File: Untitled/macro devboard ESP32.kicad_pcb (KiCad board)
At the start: 4 copper layers, 65.6 x 57.1 mm, 57 parts, among them J1 12402012E212A, J3 Conn_02x04_Odd_Even, J4 Conn_01x02_Pin, Q1 BSS84LT1G, SW1 MX_SW_HS, SW2 1825232-1, SW3 RST, SW6 MX_SW_HS, SW7 MX_SW_HS, SW8 MX_SW_HS, SW9 MX_SW_HS, U1 ESP32-C3-WROOM-02, U2 MCP73831T-2ACI_OT, U3 USBLC6-2SC6, U4 XC6210B332MR

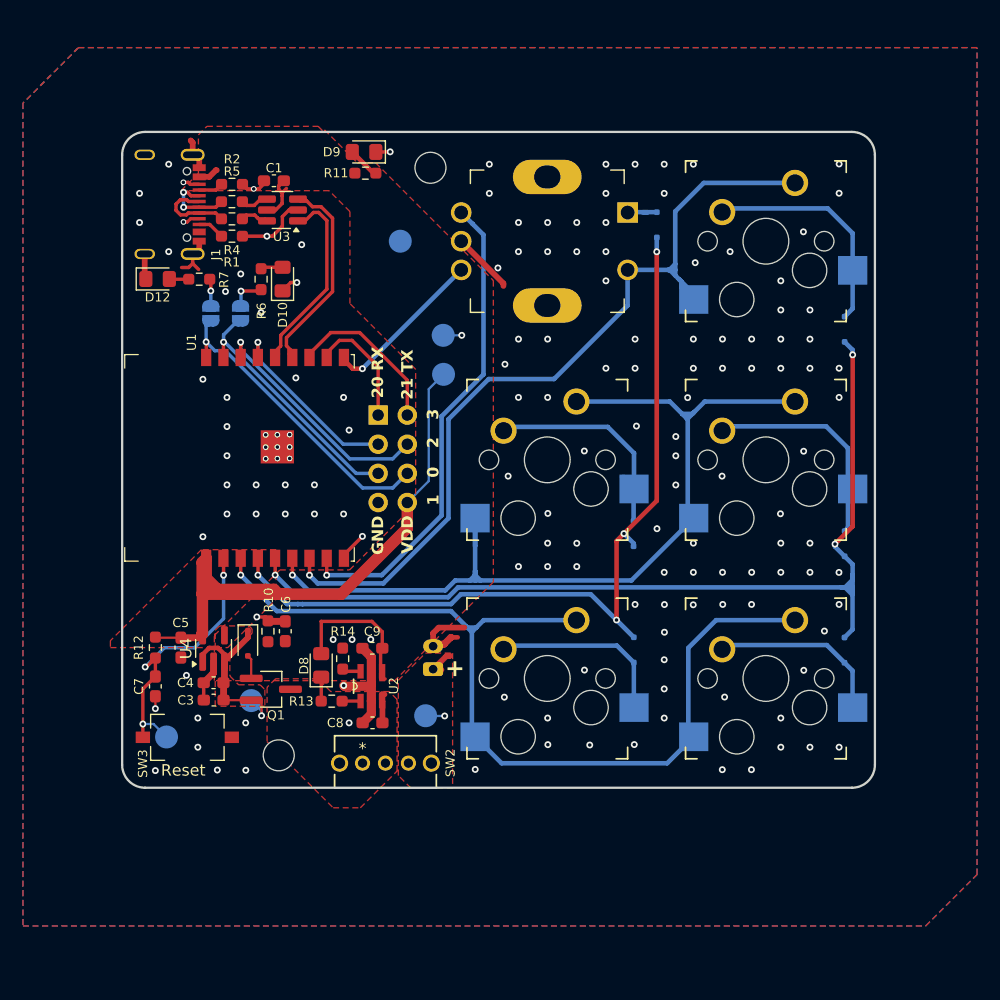
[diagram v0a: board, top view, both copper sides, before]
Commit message: this was the actual printed PCB design
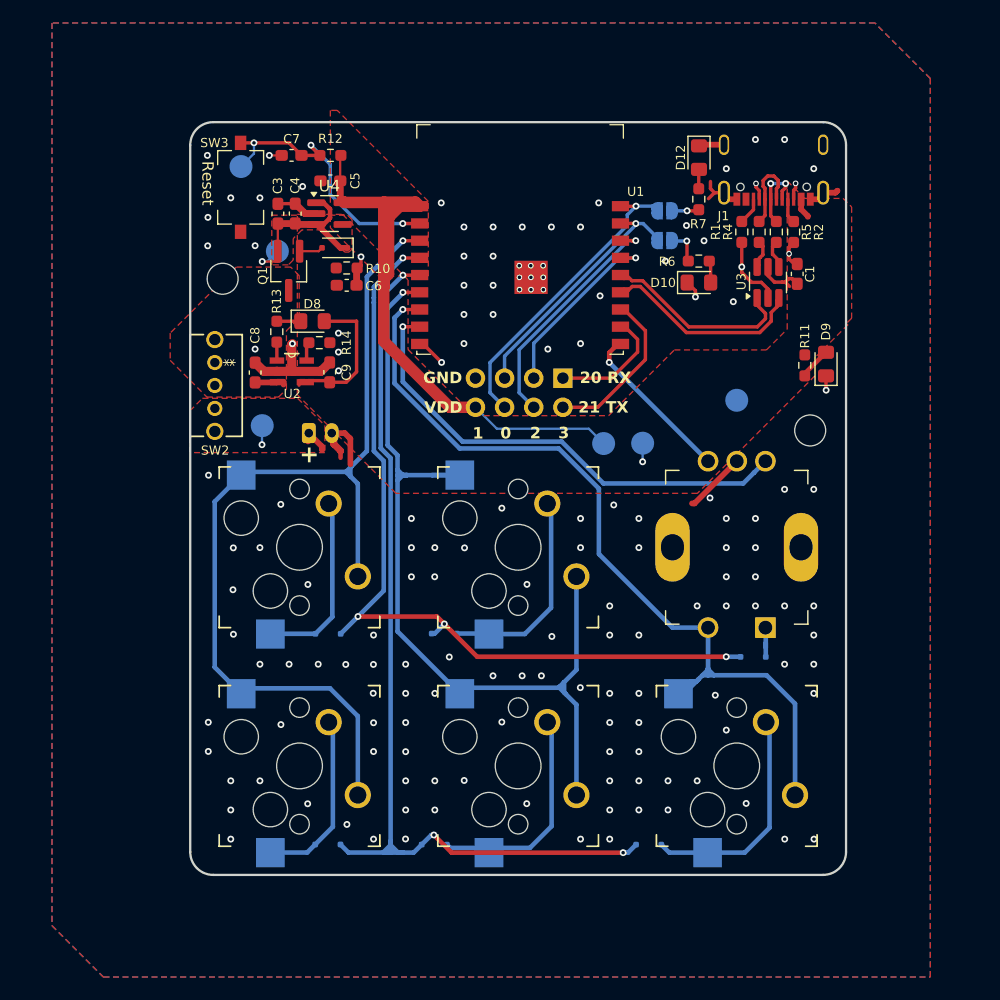
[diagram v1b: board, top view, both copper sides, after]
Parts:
- moved J1 55.0 mm to (245.8, 41.1), turned to 180 degrees
- moved TP3 50.1 mm to (199.3, 43.0), turned to -90 degrees
- moved R2 49.1 mm to (247.5, 48.7), turned to 90 degrees
- moved D12 48.3 mm to (239.3, 42.2), turned to -90 degrees
- moved SW3 48.1 mm to (199.3, 44.8), turned to 90 degrees
- moved D3 48.1 mm to (206.9, 102.1), turned to 180 degrees
- moved D2 48.0 mm to (234.9, 102.1), turned to 0 degrees
- moved C7 47.8 mm to (203.8, 42.0), turned to 0 degrees
- moved R5 47.5 mm to (246.0, 48.7), turned to 90 degrees
- moved C1 46.3 mm to (247.8, 52.4), turned to 90 degrees
- moved R4 46.0 mm to (244.5, 48.7), turned to 90 degrees
- moved SW1 45.8 mm to (242.6, 95.2), turned to -90 degrees
- moved R12 45.5 mm to (207.1, 42.0), turned to 180 degrees
- moved R1 44.4 mm to (243.0, 48.7), turned to 90 degrees
- moved D4 44.3 mm to (216.2, 102.1), turned to 0 degrees
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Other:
- board size 65.6 x 57.1 mm -> 57.1 x 65.6 mm
